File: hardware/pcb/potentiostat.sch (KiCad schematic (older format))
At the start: 16 parts

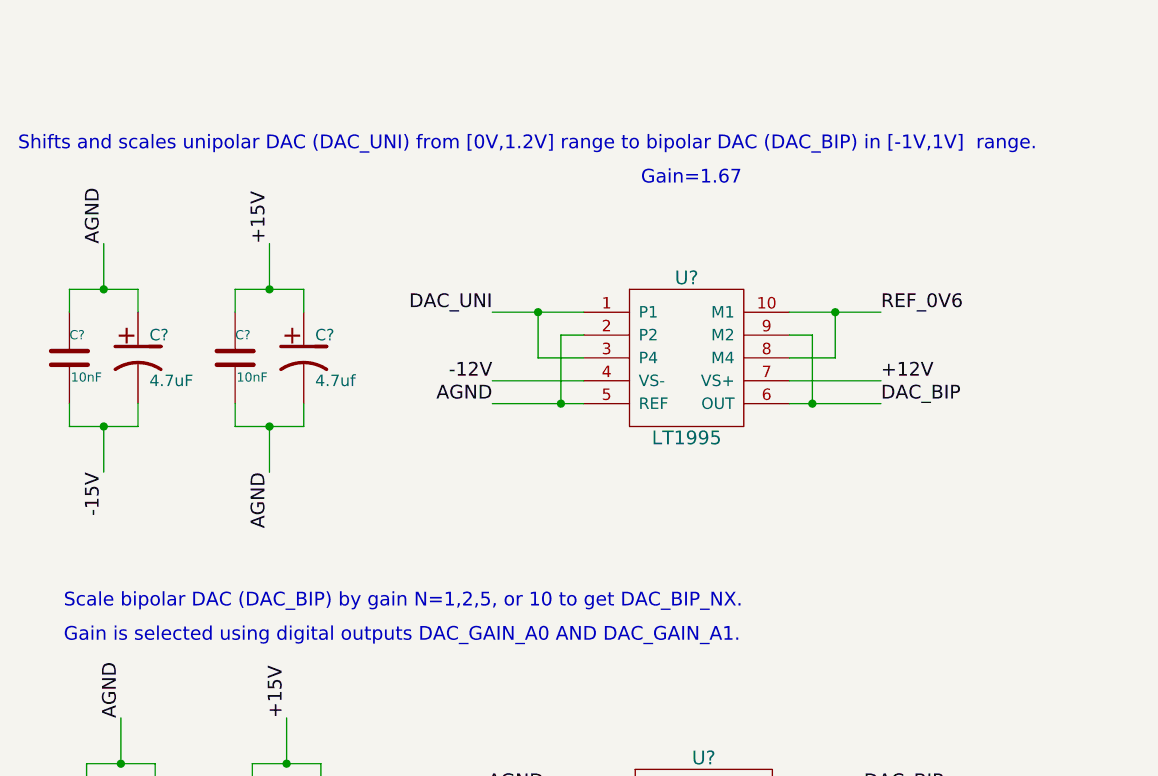
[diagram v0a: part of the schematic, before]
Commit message: More work on design.
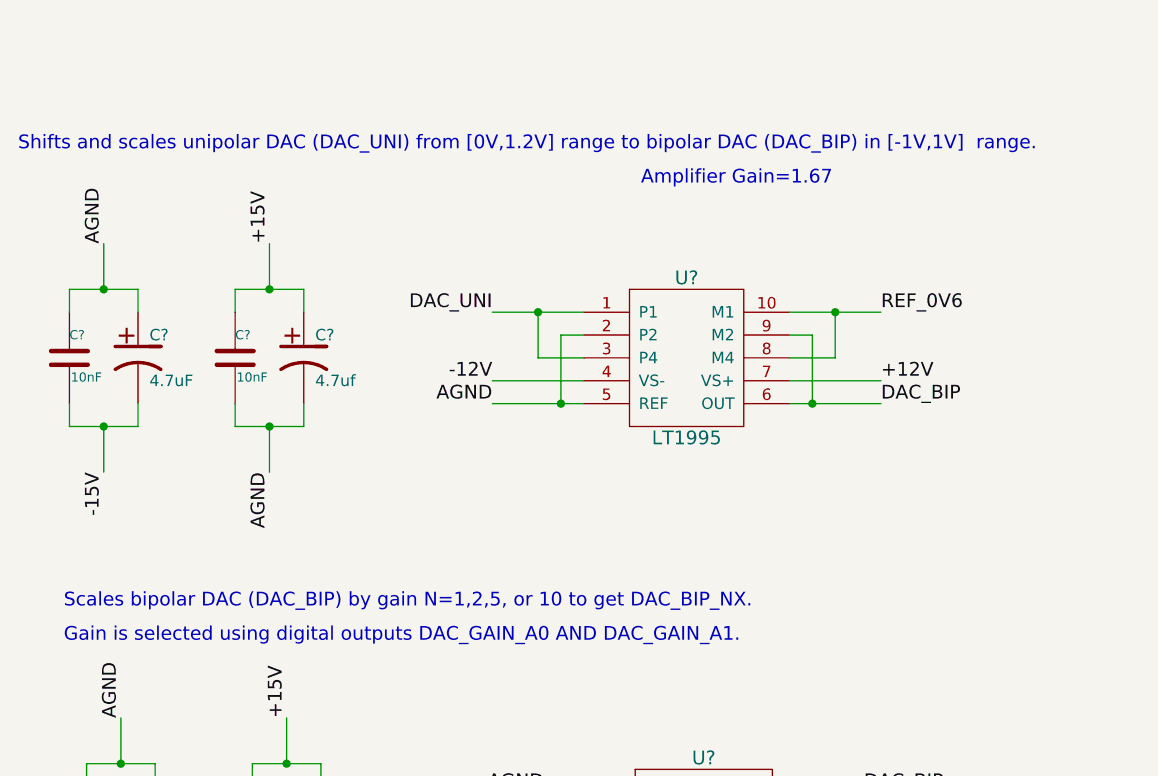
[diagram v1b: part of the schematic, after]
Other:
- note added: "Amplifier Gain=1.67"
- note added: "Scales bipolar DAC (DAC_BIP) by gain N=1,2,5, or 10 to get DAC_BIP_NX."
- note removed: "Gain=1.67"
- note removed: "Scale bipolar DAC (DAC_BIP) by gain N=1,2,5, or 10 to get DAC_BIP_NX."
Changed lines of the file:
@@
 +15V
 Text Notes 925  6700 0    60   ~ 0
-Scale bipolar DAC (DAC_BIP) by gain N=1,2,5, or 10 to get DAC_BIP_NX.
+Scales bipolar DAC (DAC_BIP) by gain N=1,2,5, or 10 to get DAC_BIP_NX.
 Text Notes 925  6850 0    60   ~ 0
 Gain is selected using digital outputs DAC_GAIN_A0 AND DAC_GAIN_A1.
@@
 +15V
 Text Notes 3450 4850 0    60   ~ 0
-Gain=1.67
+Amplifier Gain=1.67
 $Comp
 L MEA1D05XXSC U?
